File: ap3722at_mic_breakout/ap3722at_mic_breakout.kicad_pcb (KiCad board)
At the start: 2 copper layers, 20 x 20 mm, 5 parts, among them J1 Conn_01x03_Female, M201 APT3722AT

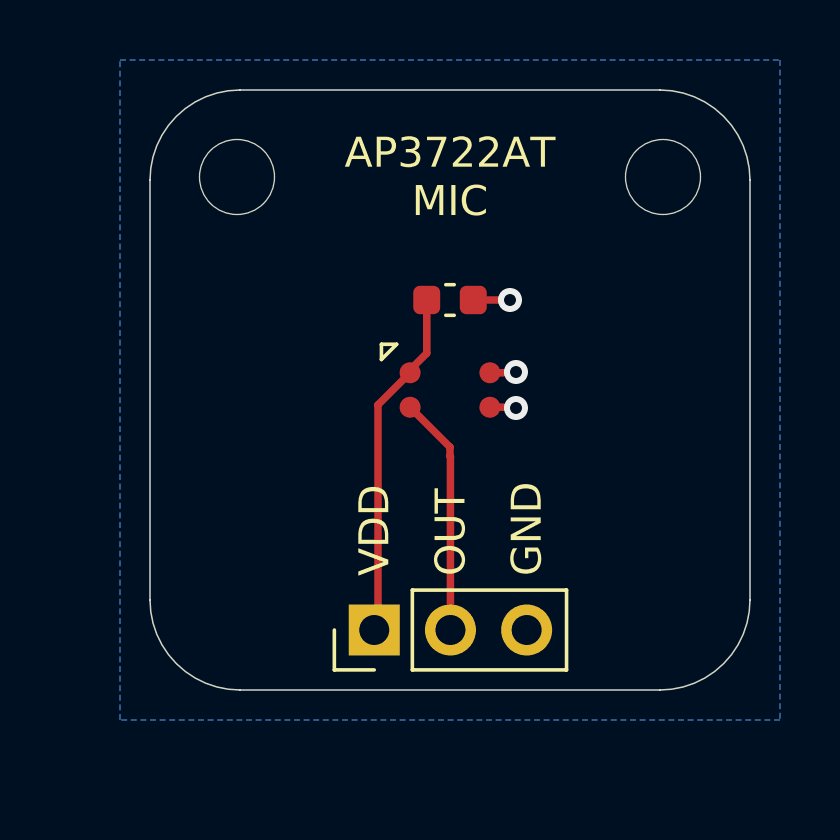
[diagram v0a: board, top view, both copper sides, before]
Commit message: final touches + v1 jlcpcb fab files
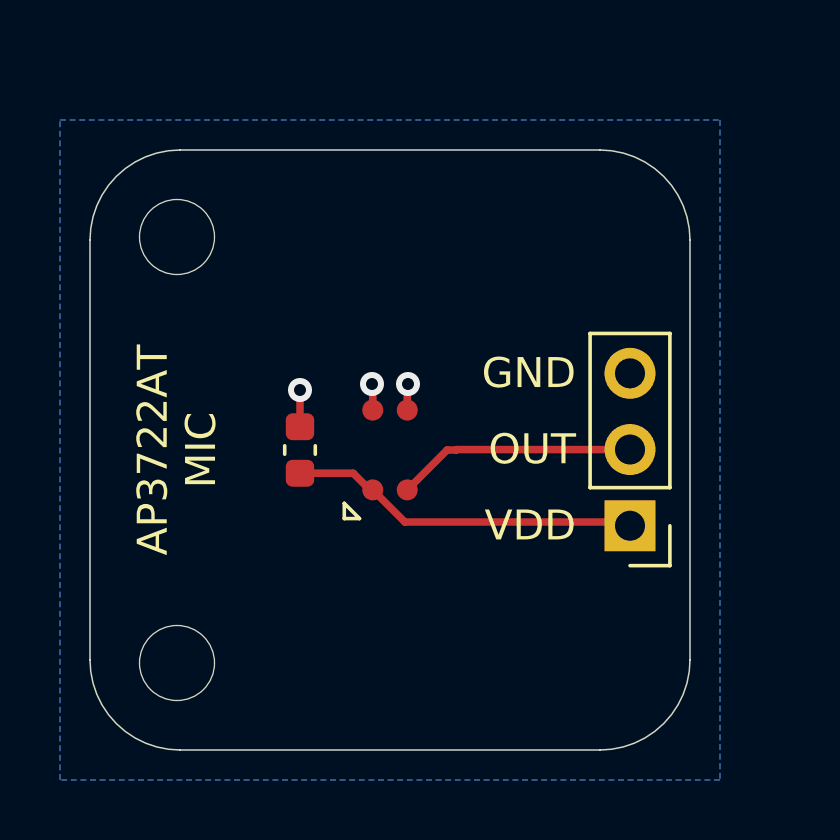
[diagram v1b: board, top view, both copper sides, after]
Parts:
- moved REF** 16.3 mm to (158.9, 120.1), turned to 90 degrees
- moved REF** 16.3 mm to (158.9, 105.9), turned to 90 degrees
- moved J1 9.21 mm to (174.0, 115.5), turned to 180 degrees
- moved C201 7.07 mm to (163.0, 113.0), turned to -90 degrees
- moved M201 2.83 mm to (166.0, 113.0), turned to 180 degrees
